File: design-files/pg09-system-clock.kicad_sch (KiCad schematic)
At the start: 10 parts, among them J201 Clock Speed, U201 CD74ACT109, U202 CD74ACT163, U204 GAL22V10, X201 ACO-32.000MHz

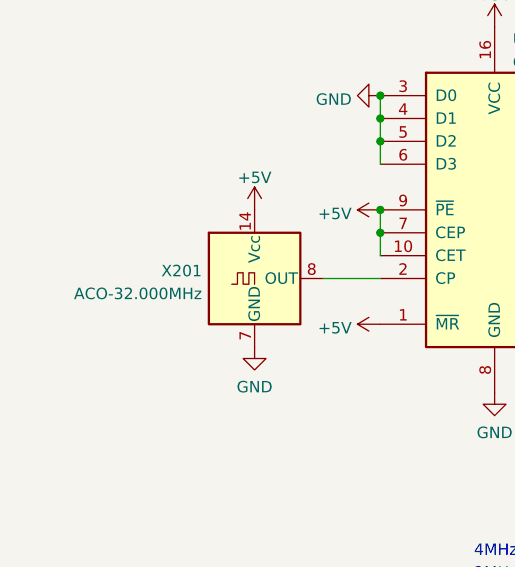
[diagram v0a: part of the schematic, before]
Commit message: Re-do the UARTs using a single TL16C2552 dual-UART in PLCC-44 package.
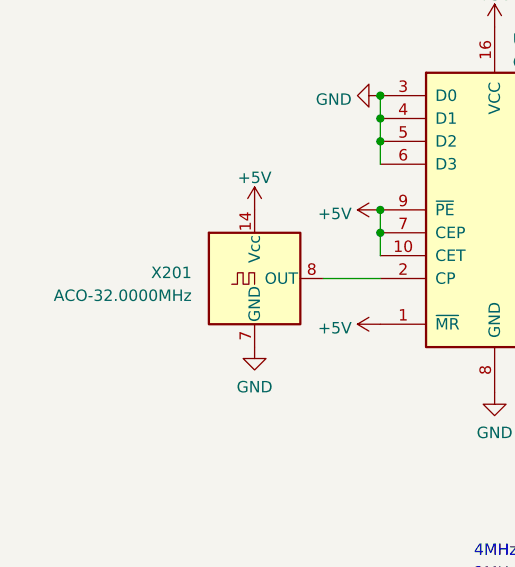
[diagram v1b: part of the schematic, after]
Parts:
- X201: value ACO-32.000MHz -> ACO-32.0000MHz
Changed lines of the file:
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@@
   (symbol (lib_id "Oscillator:ACO-xxxMHz") (at 69.215 97.155 0) (unit 1)
     (in_bom yes) (on_board yes) (dnp no) (fields_autoplaced)
-    (property "Reference" "X201" (at 63.373 96.3203 0)
+    (property "Reference" "X201" (at 62.23 96.52 0)
       (effects (font (size 1.27 1.27)) (justify right))
     )
-    (property "Value" "ACO-32.000MHz" (at 63.373 98.8572 0)
+    (property "Value" "ACO-32.0000MHz" (at 62.23 99.06 0)
       (effects (font (size 1.27 1.27)) (justify right))
     )
